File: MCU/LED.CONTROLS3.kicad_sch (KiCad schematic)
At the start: 8 parts, among them U8 HHG1D-1, U9 AMC1301DWVR

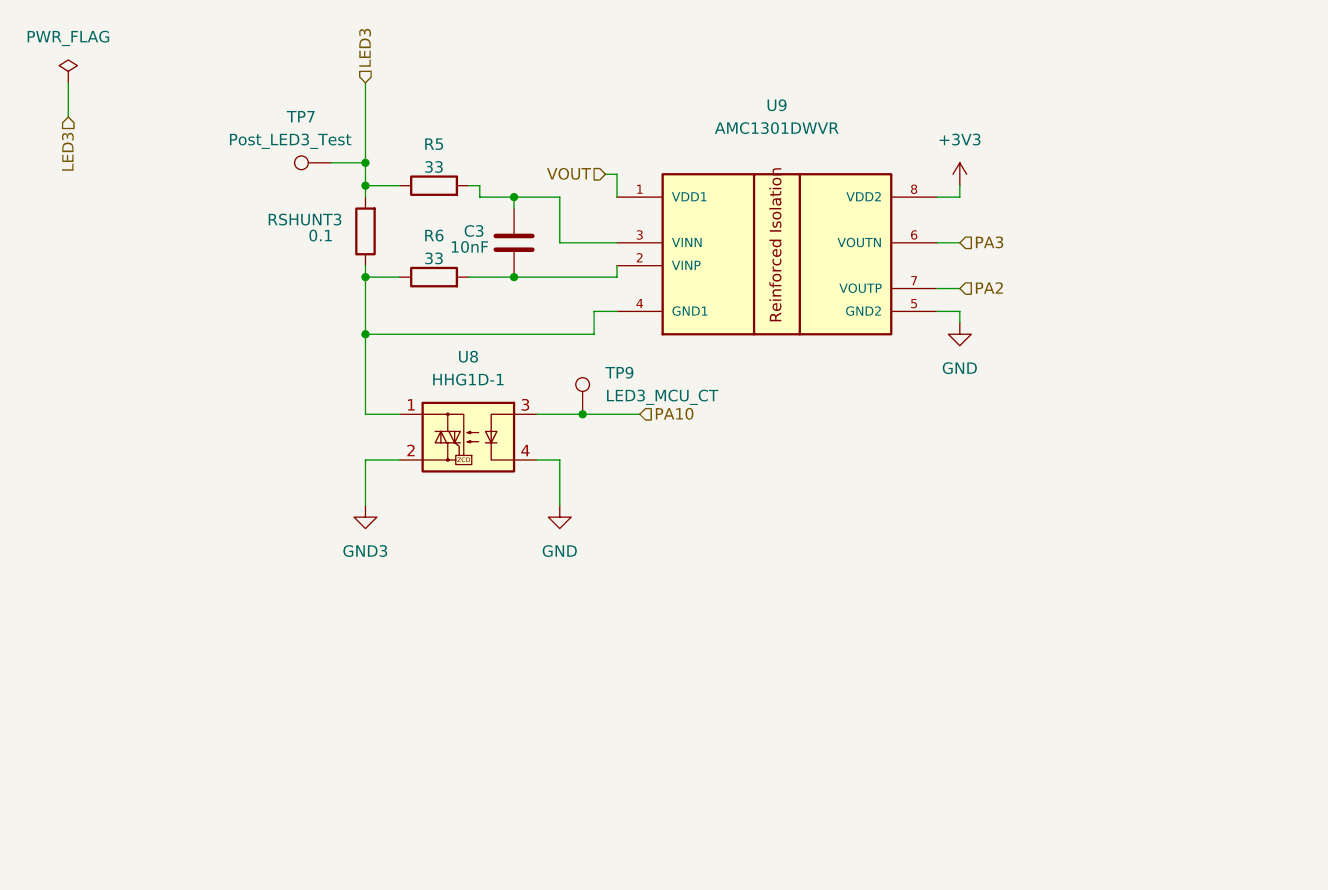
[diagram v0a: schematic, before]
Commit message: Finalized schematic and started layout
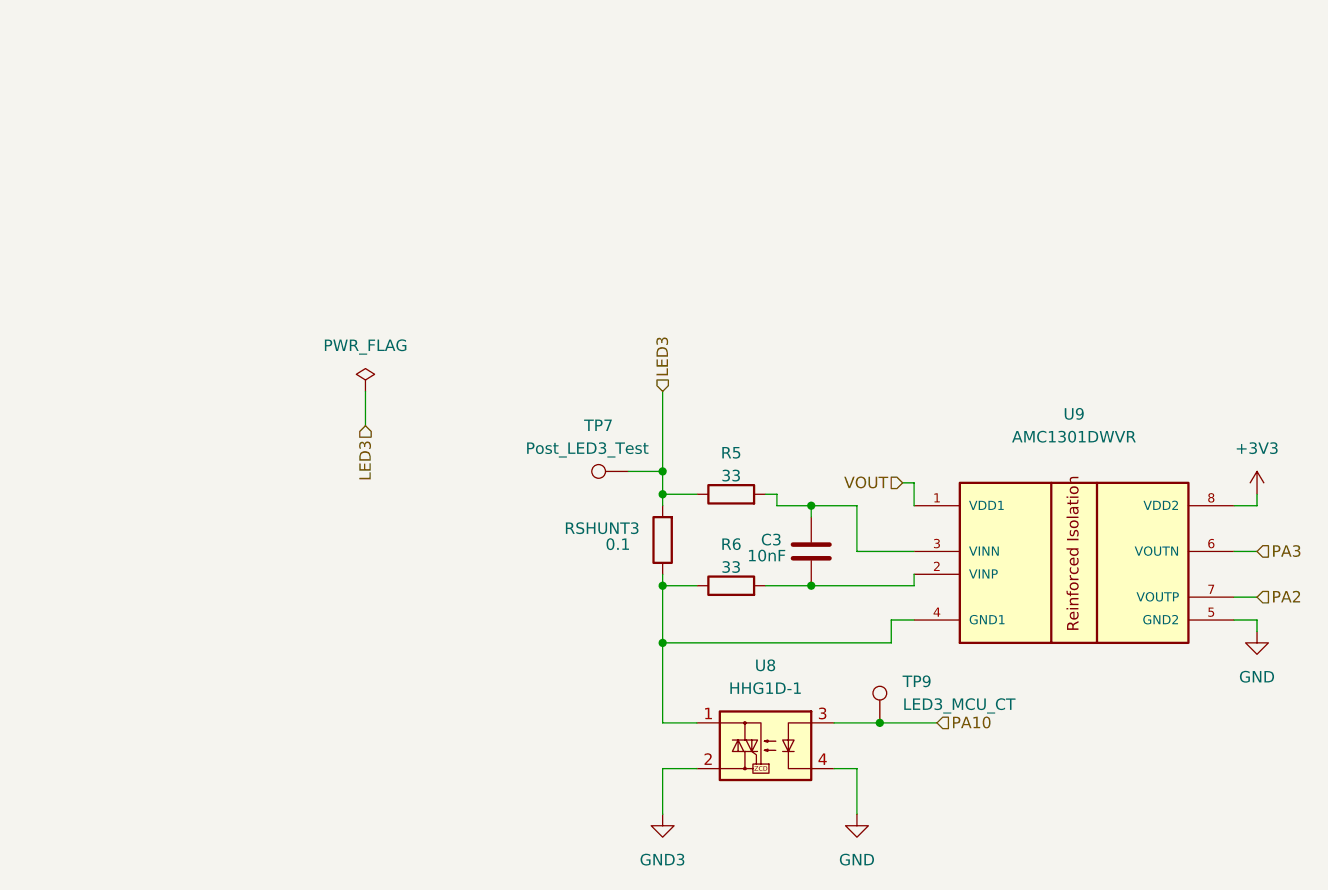
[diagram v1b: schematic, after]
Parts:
- U9: footprint AMC1301DWVR:SOIC127P1150X280-8N -> AMC1301 Isolated Amplifier:DWV0008A
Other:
- moved on the sheet: C3, R5, R6, RSHUNT3, TP7, TP9, U8, U9
